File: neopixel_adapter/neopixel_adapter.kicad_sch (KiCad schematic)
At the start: 5 parts, among them J1 Conn_01x02, J2 Conn_01x02

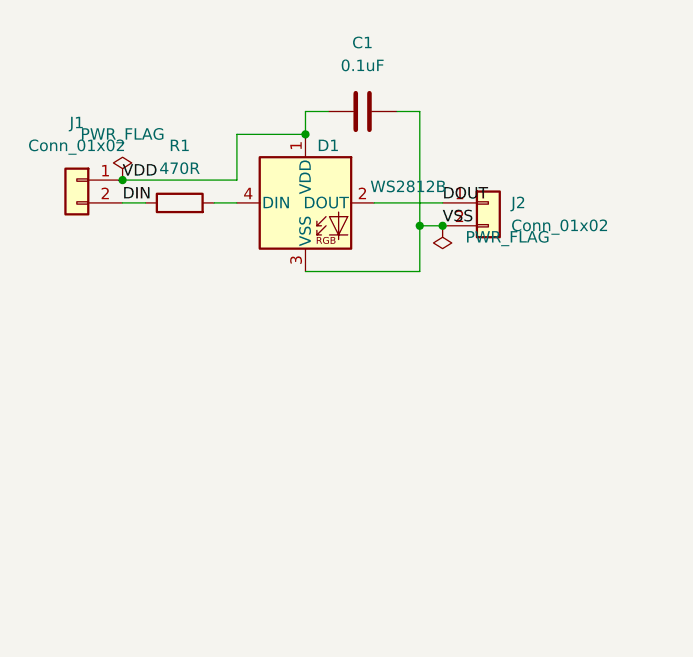
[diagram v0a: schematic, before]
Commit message: Add .gitignore.
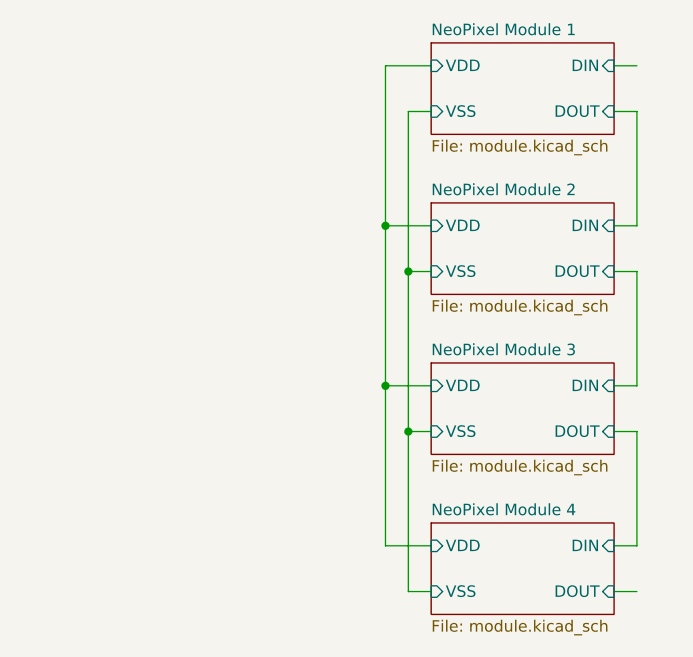
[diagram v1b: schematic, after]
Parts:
- removed C1: 0.1uF, Capacitor_SMD:C_0805_2012Metric_Pad1.18x1.45mm_HandSolder, symbol Device:C
- removed D1: WS2812B, LED_SMD:LED_WS2812B_PLCC4_5.0x5.0mm_P3.2mm, symbol LED:WS2812B
- removed J1, J2: Conn_01x02, Connector_PinHeader_2.54mm:PinHeader_1x02_P2.54mm_Vertical, symbol Connector_Generic:Conn_01x02
- removed R1: 470R, Resistor_SMD:R_0805_2012Metric_Pad1.20x1.40mm_HandSolder, symbol Device:R
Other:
- added sheet NeoPixel Module 1 (module.kicad_sch)
- added sheet NeoPixel Module 2 (module.kicad_sch)
- added sheet NeoPixel Module 3 (module.kicad_sch)
- added sheet NeoPixel Module 4 (module.kicad_sch)
